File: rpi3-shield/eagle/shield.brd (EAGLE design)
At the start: 85 x 56 mm, 8 parts, among them J1 RJ12STRAIGHT-I2C, J2 RJ12STRAIGHT-I2C, J3 RJ12STRAIGHT-I2C, J4 22-27-2061-06, J5 22-27-2061-06, J6 22-27-2061-06, J7 22-27-2061-06

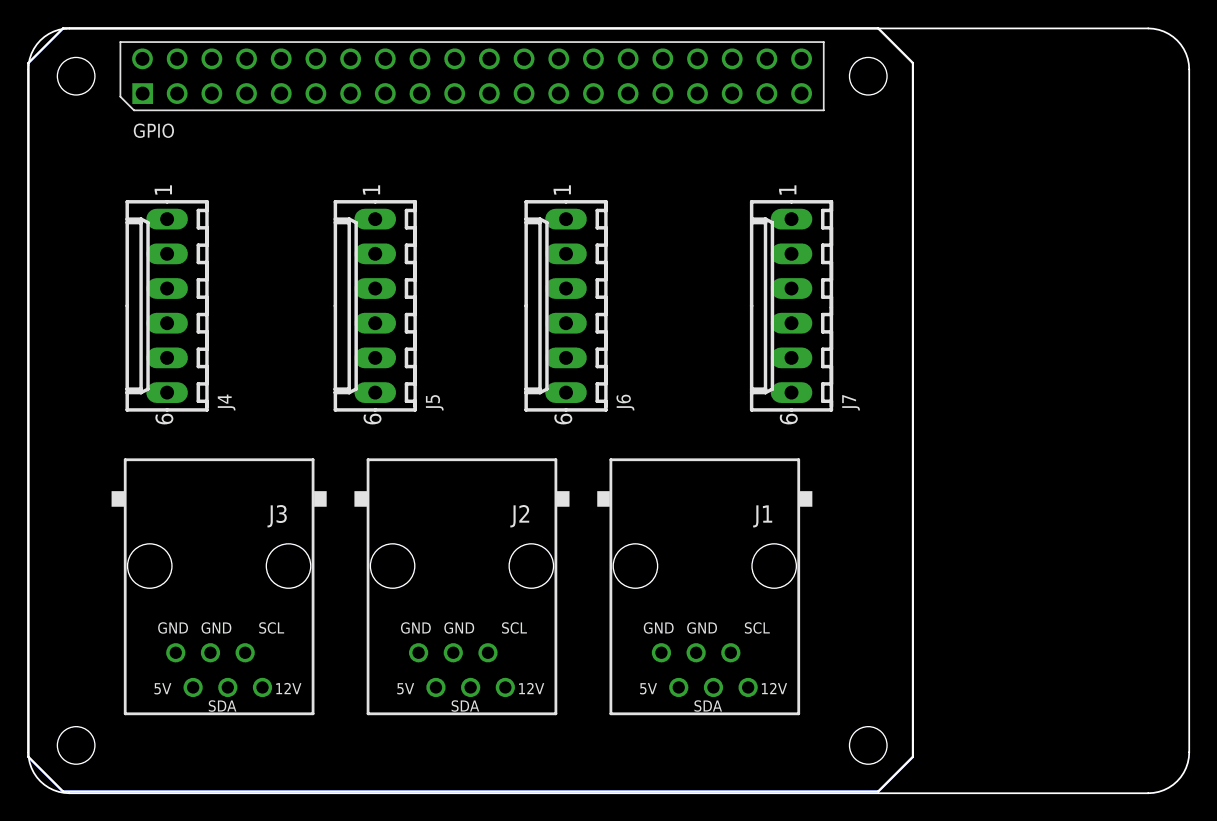
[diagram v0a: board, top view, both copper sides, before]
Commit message: rpi3-shield: v1.0.0 submitted for production
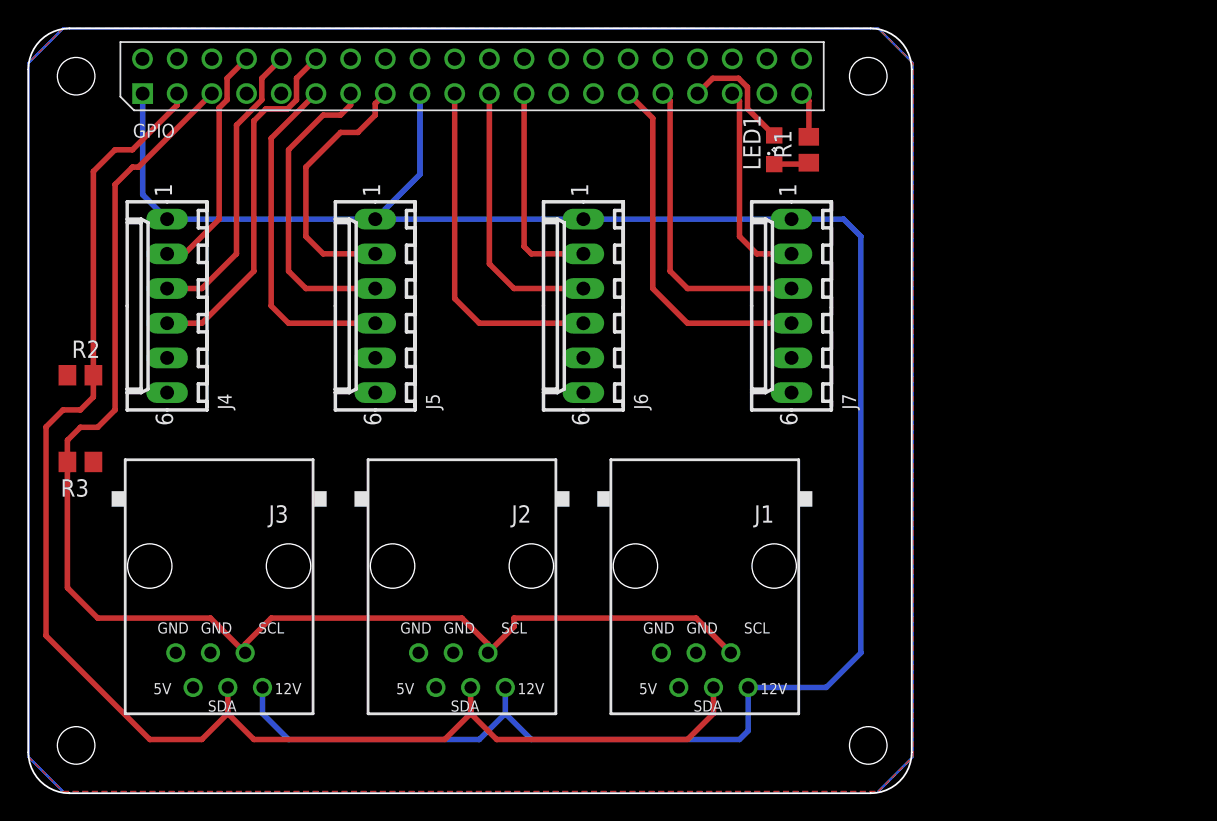
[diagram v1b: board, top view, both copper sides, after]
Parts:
- added LED1: red, led:SML0805
- added R1: 1k, rcl:R0805
- added R2, R3: 10k, rcl:R0805
- moved J6 1.27 mm to (41.9, 36.8)
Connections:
- new net IO13: LED1.A, PCB1.P$33
- new net IO17: J5.4, PCB1.P$11
- new net IO18: J4.4, PCB1.P$12
- new net IO19: J7.2, PCB1.P$35
- new net IO22: J5.2, PCB1.P$15
- new net IO27: J5.3, PCB1.P$13
- new net IO5: J7.4, PCB1.P$29
- new net IO6: J7.3, PCB1.P$31
- new net N$2: LED1.C, R1.1
- net +3V3: now also J1.+12V, J2.+12V, J3.+12V, J4.1, J5.1, J6.1, J7.1
- net +5V: now also J1.+5V, J2.+5V, J3.+5V, J4.5, J5.5, J6.5, J7.5, R2.1, R3.1
- net GND: now also J1.GND1, J1.GND2, J2.GND1, J2.GND2, J3.GND1, J3.GND2, J4.6, J5.6, J6.6, J7.6, R1.2
- net MISO0: now also J6.3
- net MOSI0: now also J6.4
- net RX: now also J4.3
- net SCL1: now also J1.SCL, J2.SCL, J3.SCL, R3.2
- net SCLK0: now also J6.2
- net SDA1: now also J1.SDA, J2.SDA, J3.SDA, R2.2
- net TX: now also J4.2
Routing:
- net +3V3: track 0.00 -> 156.8 mm
- net N$1: track 470.7 -> 351.3 mm
- net SDA1: track 0.00 -> 107.5 mm
- net SCL1: track 0.00 -> 97.4 mm
- net IO18: track 0.00 -> 26.3 mm
- net IO5: track 0.00 -> 26.2 mm
- net MOSI0: track 0.00 -> 25.2 mm
- net IO17: track 0.00 -> 25.1 mm
- net IO6: track 0.00 -> 22.6 mm
- net IO27: track 0.00 -> 22.5 mm
- net RX: track 0.00 -> 21.8 mm
- net MISO0: track 0.00 -> 20.1 mm
- net IO22: track 0.00 -> 19.2 mm
- net TX: track 0.00 -> 17.4 mm
- net SCLK0: track 0.00 -> 15.8 mm
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- added copper zone on layer 1, net +5V
- added copper zone on layer 16, net GND
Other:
- board size 85 x 56 mm -> 64.7 x 56 mm
- board text added: "17"
- board text added: "18"
- board text added: "19"
- board text added: "22"
- board text added: "27"
- board text added: "5"
- board text added: "6"
- board text added: "Legoino RPi shied v1.0.0"
- board text added: "MISO"
- board text added: "MOSI"
- board text added: "RX"
- board text added: "SCLK"
- board text added: "TX"
